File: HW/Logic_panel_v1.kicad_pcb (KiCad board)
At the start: 4 copper layers, 100.1 x 100 mm, 251 parts, among them J1 USB_B_Micro, Q1 Q_NPN_BEC, Q2 Q_NPN_BEC, Q4 Q_NMOS_GSD, Q5 Q_PMOS_GSD, Q6 Q_NMOS_GSD, Q7 Q_PMOS_GSD, Q8 Q_NMOS_GSD, Q9 Q_PMOS_GSD, SW1 SW_SPDT, SW10 button, SW11 button, SW12 button, SW2 button, SW3 button, SW4 button, SW5 button, SW6 button, SW7 button, SW8 button, SW9 button, U1 ESP32-PICO-D4, U2 CP2102N-A01-GQFN28, U3 SY8105

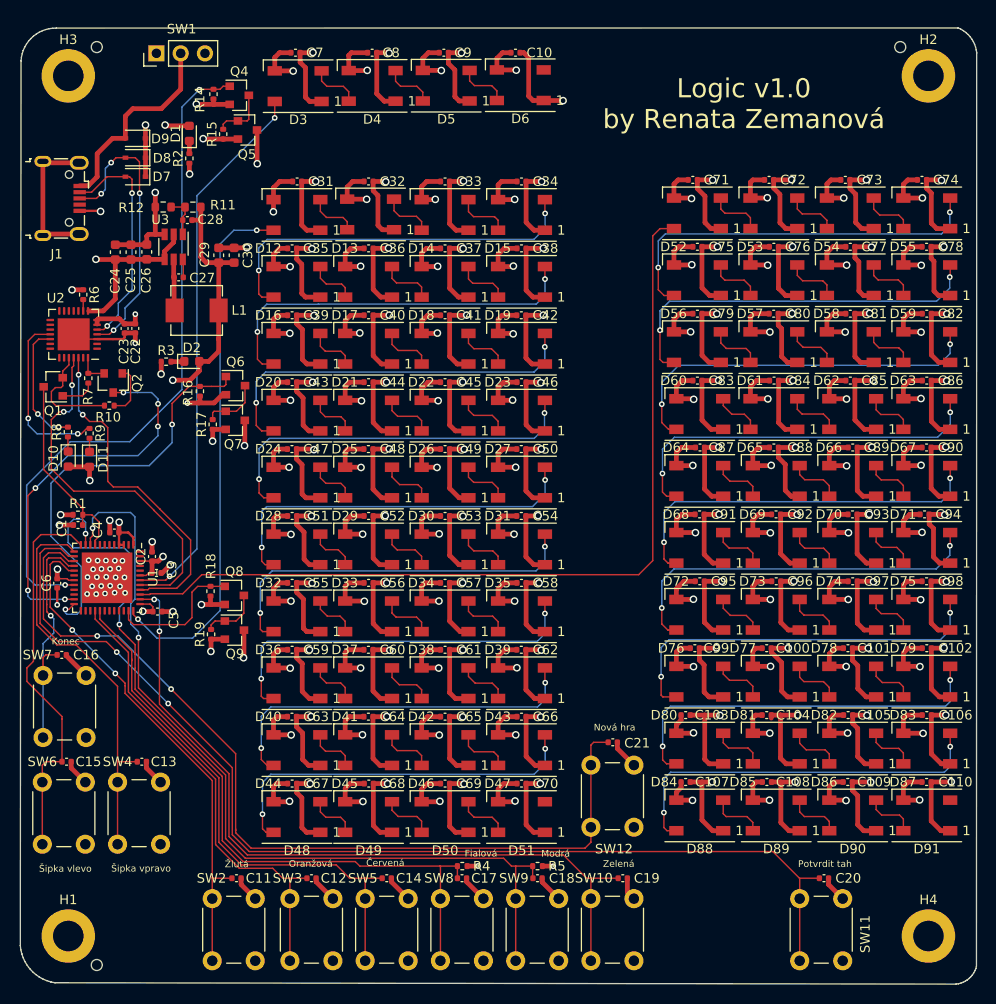
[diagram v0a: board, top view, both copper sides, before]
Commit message: v1.0 for fab
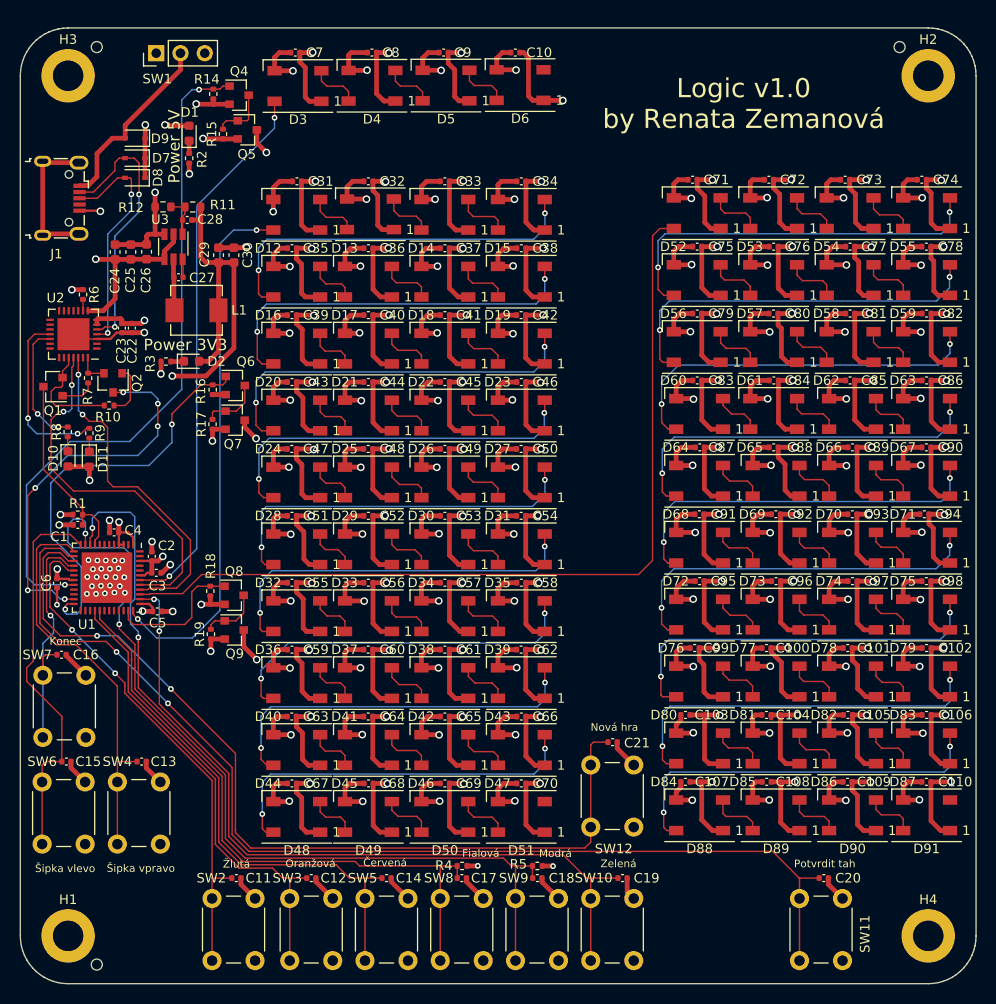
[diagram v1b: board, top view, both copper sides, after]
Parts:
- removed the REF** at (58.0, 148.0)
- removed the REF** at (142.1, 52.0)
- added REF**: NPTH, NPTH, F.Cu at (58.0, 148.0)
- added REF**: NPTH, NPTH, F.Cu at (142.0, 52.0)
- moved D8 2.11 mm to (62.0, 65.7)
- moved D7 1.95 mm to (62.0, 63.6)
- moved R16 1.35 mm to (70.1, 87.9)
- moved C22 0.36 mm to (61.7, 81.4)
- moved C23 0.28 mm to (60.6, 81.4)
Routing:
- net Board_1-+3V3: track 56.4 -> 69.1 mm
- net Board_1-Net-(D8-Pad2): track 30.2 -> 24.7 mm, vias 4 -> 2
- net Board_1-Net-(D7-Pad2): track 23.9 -> 28.6 mm
- net Board_1-GND: track 518.0 -> 514.4 mm, vias 123 -> 122
- net Board_1-V_IN: track 21.3 -> 19.5 mm
- net Board_1-/herni_LED.sch/8.sch/DATA_IN: track 40.2 -> 38.8 mm
- net Board_1-V_LED_3: track 206.6 -> 207.4 mm
- net Board_1-V_LED_1: track 302.1 -> 301.3 mm
- net Board_1-ZAPINANI_2_CAST_LED: track 43.8 -> 43.2 mm
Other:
- board size 100.1 x 100 mm -> 100 x 100 mm
- board text added: "Power 3V3"
- board text added: "Power 5V"
